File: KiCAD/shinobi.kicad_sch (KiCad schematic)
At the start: 111 parts, among them IC1 TPS62825DMQT, IC2 TPS62825DMQT, IC3 74LVC2G17GW-Q100H, J2 61300711121, J3 61301011121, J4 61300211121, J5 USB_C_Receptacle_USB2.0_16P, Q1 UMH3N, U1 TV5725, U2 W9864G2JH-6, U5 SI5351A, U6 CH343P, U7 ESP8285, Y1 CRYSTAL2.5X2.0, Y2 CRYSTAL2.5X2.0, Y3 26MHz

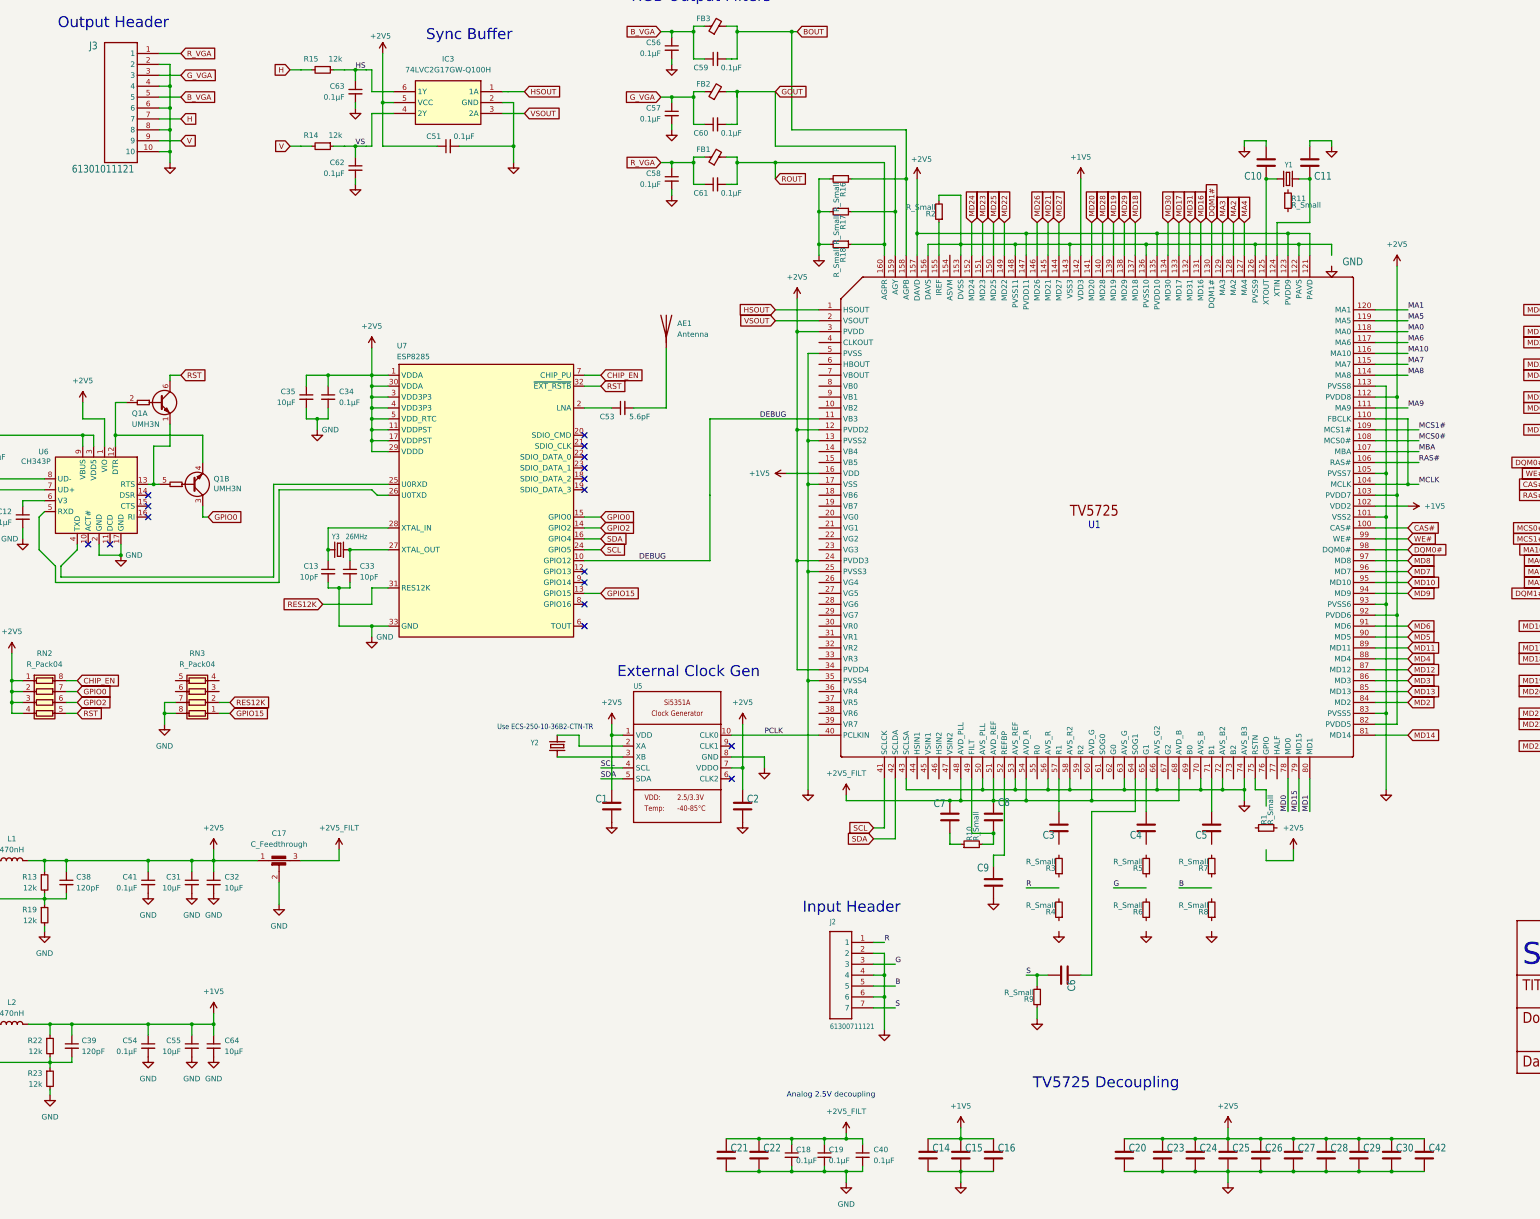
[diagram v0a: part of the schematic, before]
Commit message: shinobi2 routing
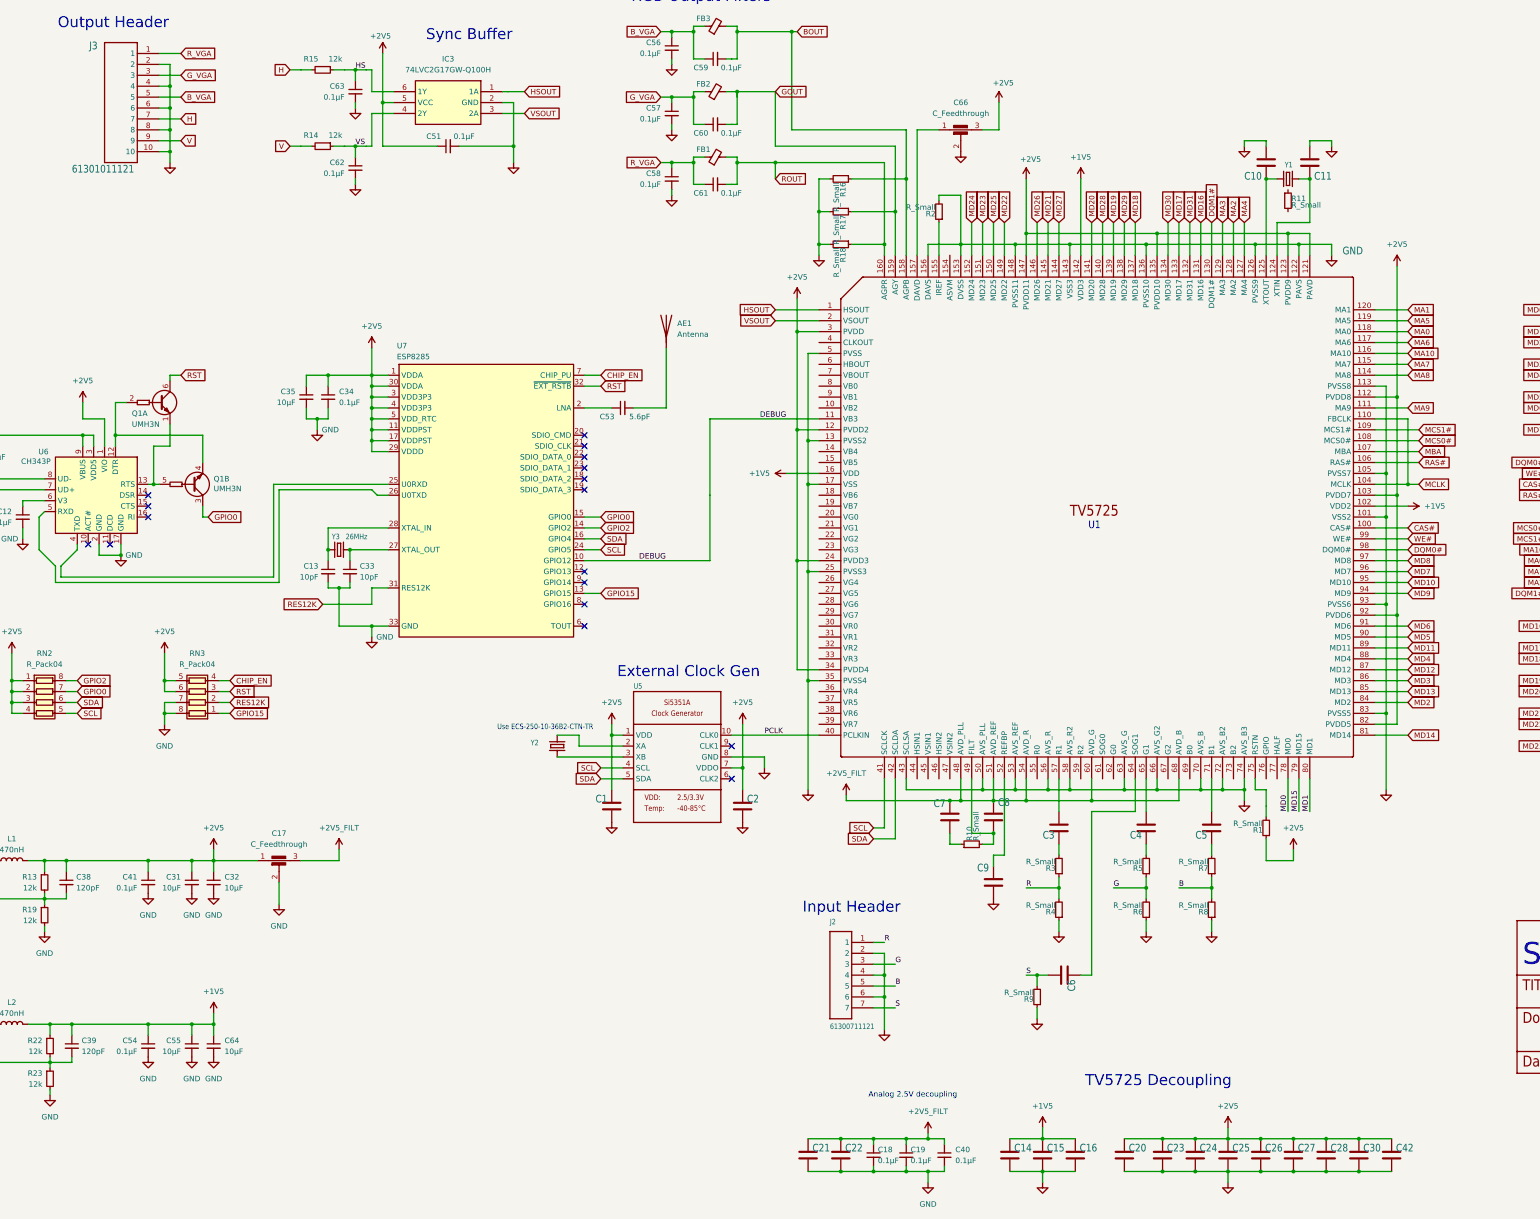
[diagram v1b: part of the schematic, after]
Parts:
- removed C29: C-USC0402, Capacitor_SMD:C_0402_1005Metric, symbol Device:C
- added C66: C_Feedthrough, SamacSys_Parts:NFM18PC106D0J3L, symbol Device:C_Feedthrough
- Y1, Y2, Y3: footprint Crystal:Crystal_SMD_2520-4Pin_2.5x2.0mm -> SamacSys_Parts:Crystal_SMD_2520-4Pin_2.5x2.0mm
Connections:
- net +2V5: now also R1.1, RN3.5 (R4.2), RN3.6 (R3.2), C66.3; no longer U1.157 (DAVD)
- net B: now also R7.1, R8.2
- net CHIP_EN: now also RN3.4 (R4.1); no longer RN2.8 (R1.2)
- net G: now also R5.1, R6.2
- net GND: now also R2.2, R4.1, R6.1, R8.1, U1.122 (PAVS), U1.126 (PVSS9), U1.136 (PVSS10), U1.143 (VSS3), U1.148 (PVSS11), U1.153 (DVSS), U1.156 (DAVS), C66.2, C66.4
- net GPIO2: now also RN2.8 (R1.2); no longer RN2.6 (R3.2)
- net R: now also R3.1, R4.2
- net RST: now also RN3.3 (R3.1); no longer RN2.5 (R4.2)
- net SCL: now also RN2.5 (R4.2)
- net SDA: now also RN2.6 (R3.2)
- net at R3.2: now also C3.1
- net at U1.75 (RSTN): now also R1.2
- net at R5.2: now also C4.1
- net at C5.1: now also R7.2
- new net: C66.1, U1.157 (DAVD)
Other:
- moved on the sheet: C14, C15, C16, C18, C19, C21, C22, C30, C40, C42, R1

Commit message: Update PCB and BOM
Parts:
- AE1: value Antenna -> AMCA72-2R470G-S1F-T4
- C18: renamed from C63; value 0.1μF -> 130pF
- C19: renamed from C62; value 0.1μF -> 130pF
- C20: renamed from C17; value C_Feedthrough -> NFM18PC106D0J3L
- C22: renamed from C1; value C-USC0402 -> 0.1μF
- C24: renamed from C56; value 0.1μF -> 47pF
- C25: renamed from C57; value 0.1μF -> 47pF
- C26: renamed from C58; value 0.1μF -> 47pF
- C27: renamed from C59; value 0.1μF -> 15pF
- C28: renamed from C60; value 0.1μF -> 15pF
- C29: renamed from C61; value 0.1μF -> 15pF
- C30: renamed from C2; value C-USC0402 -> 0.1μF
- C31: renamed from C21; value C-USC0402 -> 0.1μF
- C32: renamed from C22; value C-USC0402 -> 0.1μF
- C36: renamed from C7; value C-USC0402 -> 47nF
- C37: renamed from C66; value C_Feedthrough -> NFM18PC106D0J3L
- C38: renamed from C8; value C-USC0402 -> 47nF
- C39: renamed from C9; value C-USC0402 -> 47nF
- C40: renamed from C14; value C-USC0402 -> 0.1μF
- C41: renamed from C15; value C-USC0402 -> 0.1μF
- C42: renamed from C3; value C-USC0402 -> 47nF
- C43: renamed from C6; value C-USC0402 -> 1nF
- C44: renamed from C16; value C-USC0402 -> 0.1μF
- C45: renamed from C20; value C-USC0402 -> 0.1μF
- C46: renamed from C4; value C-USC0402 -> 47nF
- C47: renamed from C23; value C-USC0402 -> 0.1μF
- C48: renamed from C24; value C-USC0402 -> 0.1μF
- C49: renamed from C5; value C-USC0402 -> 47nF
- C50: renamed from C25; value C-USC0402 -> 0.1μF
- C51: renamed from C26; value C-USC0402 -> 0.1μF
- C52: renamed from C10; value C-USC0402 -> 15pF
- C53: renamed from C27; value C-USC0402 -> 0.1μF
- C54: renamed from C11; value C-USC0402 -> 15pF
- C55: renamed from C28; value C-USC0402 -> 0.1μF
- C56: renamed from C30; value C-USC0402 -> 0.1μF
- C57: renamed from C42; value C-USC0402 -> 0.1μF
- C58: renamed from C43; value C-USC0402 -> 0.1μF
- C59: renamed from C44; value C-USC0402 -> 0.1μF
- C60: renamed from C45; value C-USC0402 -> 0.1μF
- C61: renamed from C46; value C-USC0402 -> 0.1μF
- C62: renamed from C47; value C-USC0402 -> 0.1μF
- C63: renamed from C48; value C-USC0402 -> 0.1μF
- C64: renamed from C49; value C-USC0402 -> 0.1μF
- C65: renamed from C50; value C-USC0402 -> 0.1μF
- FB1: renamed from FB3; value FerriteBead_Small -> BLM15BD221SN1D; footprint (none) -> Inductor_SMD:L_0402_1005Metric
- FB2: value FerriteBead_Small -> BLM15BD221SN1D; footprint (none) -> Inductor_SMD:L_0402_1005Metric
- FB3: renamed from FB1; value FerriteBead_Small -> BLM15BD221SN1D; footprint (none) -> Inductor_SMD:L_0402_1005Metric
- J2: renamed from J5; value USB_C_Receptacle_USB2.0_16P -> 217179-0001
- J4: renamed from J2; footprint shinobi:61300711121 -> shinobi:61300711121_11687645
- Q1: value UMH3N -> PUMH13-QF
- R10: renamed from R17; value R_Small -> 75Ω
- R11: renamed from R18; value R_Small -> 75Ω
- R12: renamed from R2; value R_Small -> 150Ω
- R13: renamed from R10; value R_Small -> 3kΩ
- R14: renamed from R9; value R_Small -> 75Ω
- R15: renamed from R3; value R_Small -> 200Ω
- R16: renamed from R4; value R_Small -> 75Ω
- R17: renamed from R5; value R_Small -> 200Ω
- R18: renamed from R6; value R_Small -> 75Ω
- R19: renamed from R7; value R_Small -> 200Ω
- R20: renamed from R8; value R_Small -> 75Ω
- R21: renamed from R1; value R_Small -> 4.7kΩ
- R22: renamed from R11; value R_Small -> 1MΩ
- R3: renamed from R13; value 12k -> 316kΩ
- R4: renamed from R19; value 12k -> 100kΩ
- R5: renamed from R22; value 12k -> 150kΩ
- R6: renamed from R23; value 12k -> 100kΩ
- R7: renamed from R15; value 12k -> 33Ω
- R8: renamed from R14; value 12k -> 33Ω
- R9: renamed from R16; value R_Small -> 75Ω
- RN1: renamed from RN2; value R_Pack04 -> EXB-28V123JX
- RN2: renamed from RN3; value R_Pack04 -> EXB-28V123JX
- U1: renamed from IC2; value TPS62825DMQT -> TPS62825DMQR; Mouser Part Number 595-TPS62825DMQT -> TPS62825DMQR
- U2: renamed from IC1; value TPS62825DMQT -> TPS62825DMQR; Mouser Part Number 595-TPS62825DMQT -> TPS62825DMQR
- Y1: renamed from Y3; value 26MHz -> ECS-260-7-36B-CKY-TR
- Y2: value CRYSTAL2.5X2.0 -> ECS-250-10-36B2-CTN-TR
- Y3: renamed from Y1; value CRYSTAL2.5X2.0 -> 830108208409
- renumbered C37 to C1, C31 to C10, C55 to C11, C35 to C12, C32 to C13, C64 to C14, C34 to C15, C13 to C16, C33 to C17, C65 to C2, C51 to C21, C53 to C23, C36 to C3, C18 to C33, C19 to C34, C40 to C35, C52 to C4, C12 to C5, C38 to C6, C39 to C7, C41 to C8, C54 to C9, J4 to J1, R20 to R1, R21 to R2, U6 to U3, U7 to U4, IC3 to U5, U5 to U6, U1 to U7, U2 to U8
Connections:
- net at C54.2, U7.124 (XTIN), Y3.3 (2): now also R22.2
- net at C52.2, U7.125 (XTOUT), Y3.1: now also R22.1
- no-connect marks 21 -> 61
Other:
- note added: "ESP8285"
- note added: "Regulators"
- note added: "USB-C to Serial"
- note removed: "U1"
- moved on the sheet: C1, C10, C11, C13, C14, C2, C20, C6, C7, C8, C9, L1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

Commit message: wip
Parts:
- C16, C17: value 10pF -> 15pF
- C6, C7: value 120pF -> 130pF
- Y1: value ECS-260-7-36B-CKY-TR -> 26MHz 10pF 2520
- Y2: value ECS-250-10-36B2-CTN-TR -> 25MHz 10pF 2520
- Y3: value 830108208409 -> 27MHz 10pF 2520
